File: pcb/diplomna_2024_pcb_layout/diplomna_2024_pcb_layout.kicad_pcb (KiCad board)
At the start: 4 copper layers, 10 parts

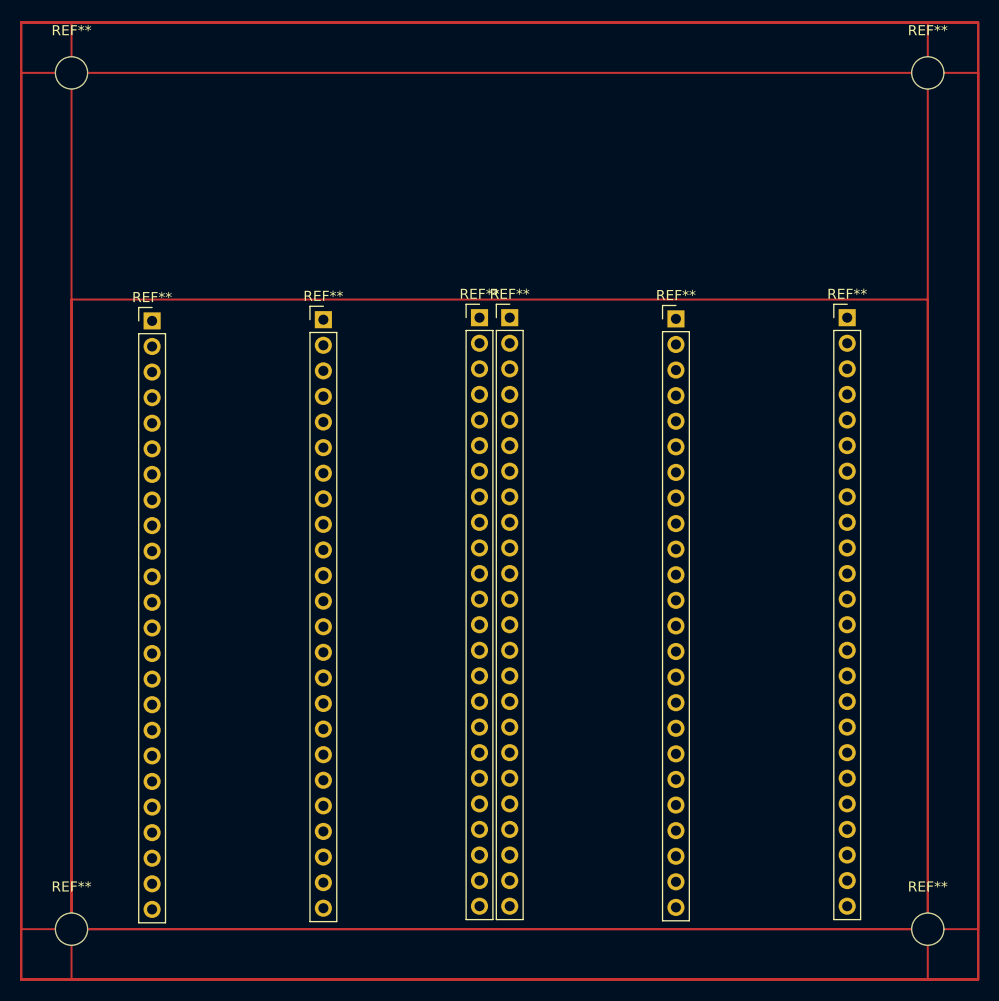
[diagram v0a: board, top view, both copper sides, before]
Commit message: pcb
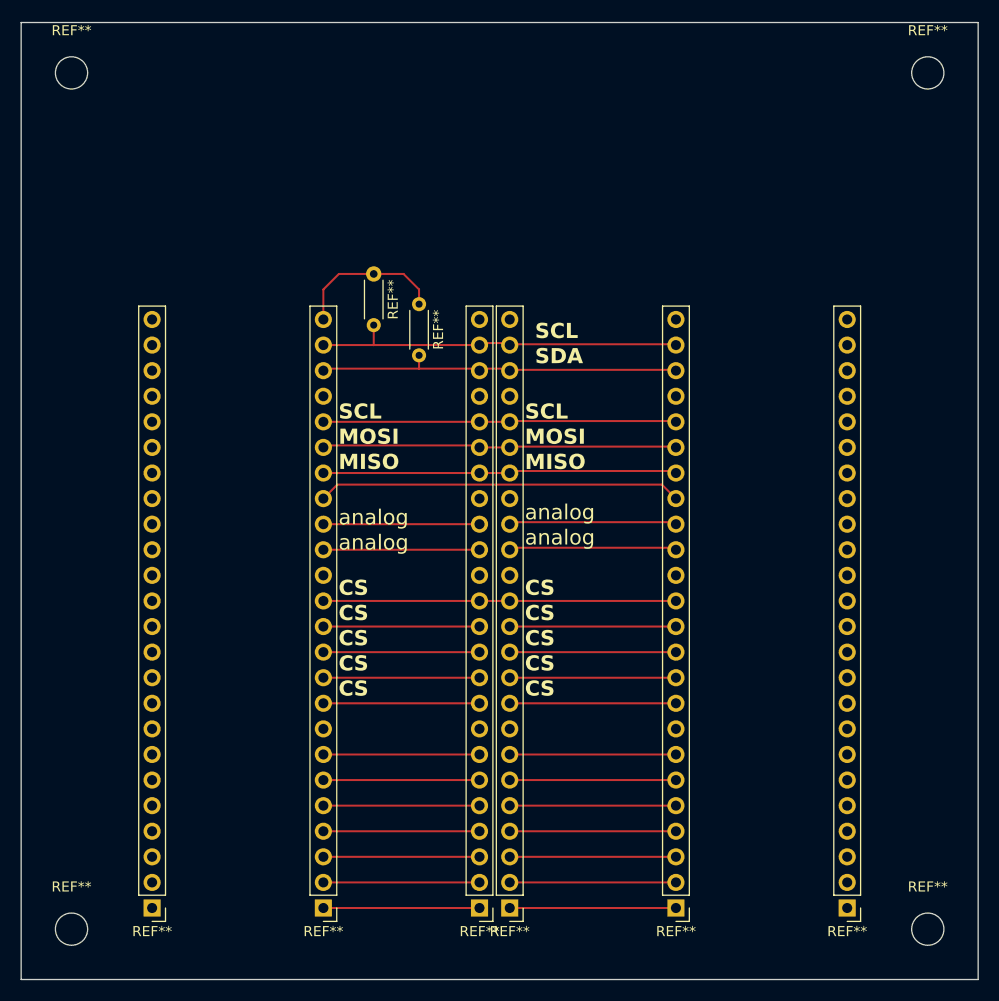
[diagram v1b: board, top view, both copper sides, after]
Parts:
- added REF**: R_Axial_DIN0204_L3.6mm_D1.6mm_P5.08mm_Horizontal, Resistor_THT:R_Axial_DIN0204_L3.6mm_D1.6mm_P5.08mm_Horizontal, F.Cu at (191.0, 75.5)
- added REF**: R_Axial_DIN0204_L3.6mm_D1.6mm_P5.08mm_Horizontal, Resistor_THT:R_Axial_DIN0204_L3.6mm_D1.6mm_P5.08mm_Horizontal, F.Cu at (195.5, 78.5)
- moved REF** 58.6 mm to (238.0, 138.4), turned to 180 degrees
- moved REF** 58.6 mm to (204.5, 138.4), turned to 180 degrees
- moved REF** 58.6 mm to (201.5, 138.4), turned to 180 degrees
- moved REF** 58.5 mm to (221.0, 138.4), turned to 180 degrees
- moved REF** 58.4 mm to (186.0, 138.4), turned to 180 degrees
- moved REF** 58.3 mm to (169.0, 138.4), turned to 180 degrees
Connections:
- REF** pad 17: (no net) -> CS (x2)
- REF** pad 24: (no net) -> VDD
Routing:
- net (no net): track 0.00 -> 632.6 mm
- net CS: track 0.00 -> 36.3 mm
- net VDD: track 0.00 -> 15.2 mm
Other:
- board outline added: 95 x 95 mm
- board text added: "CS"
- board text added: "MISO"
- board text added: "MOSI"
- board text added: "SCL"
- board text added: "SDA"
- board text added: "analog"
